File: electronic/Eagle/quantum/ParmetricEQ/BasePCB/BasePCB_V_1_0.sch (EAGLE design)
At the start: 62 parts, among them IC1 OP275_SOIC8, IC2 OP275_SOIC8, IC3 OP275_SOIC8, IC4 DAC084S085CIMM_NOPB, J1 90814-0204, J2 90814-0204, U1 THAT2181SO8-US, U2 THAT2181SO8-US, U3 THAT2181SO8-US

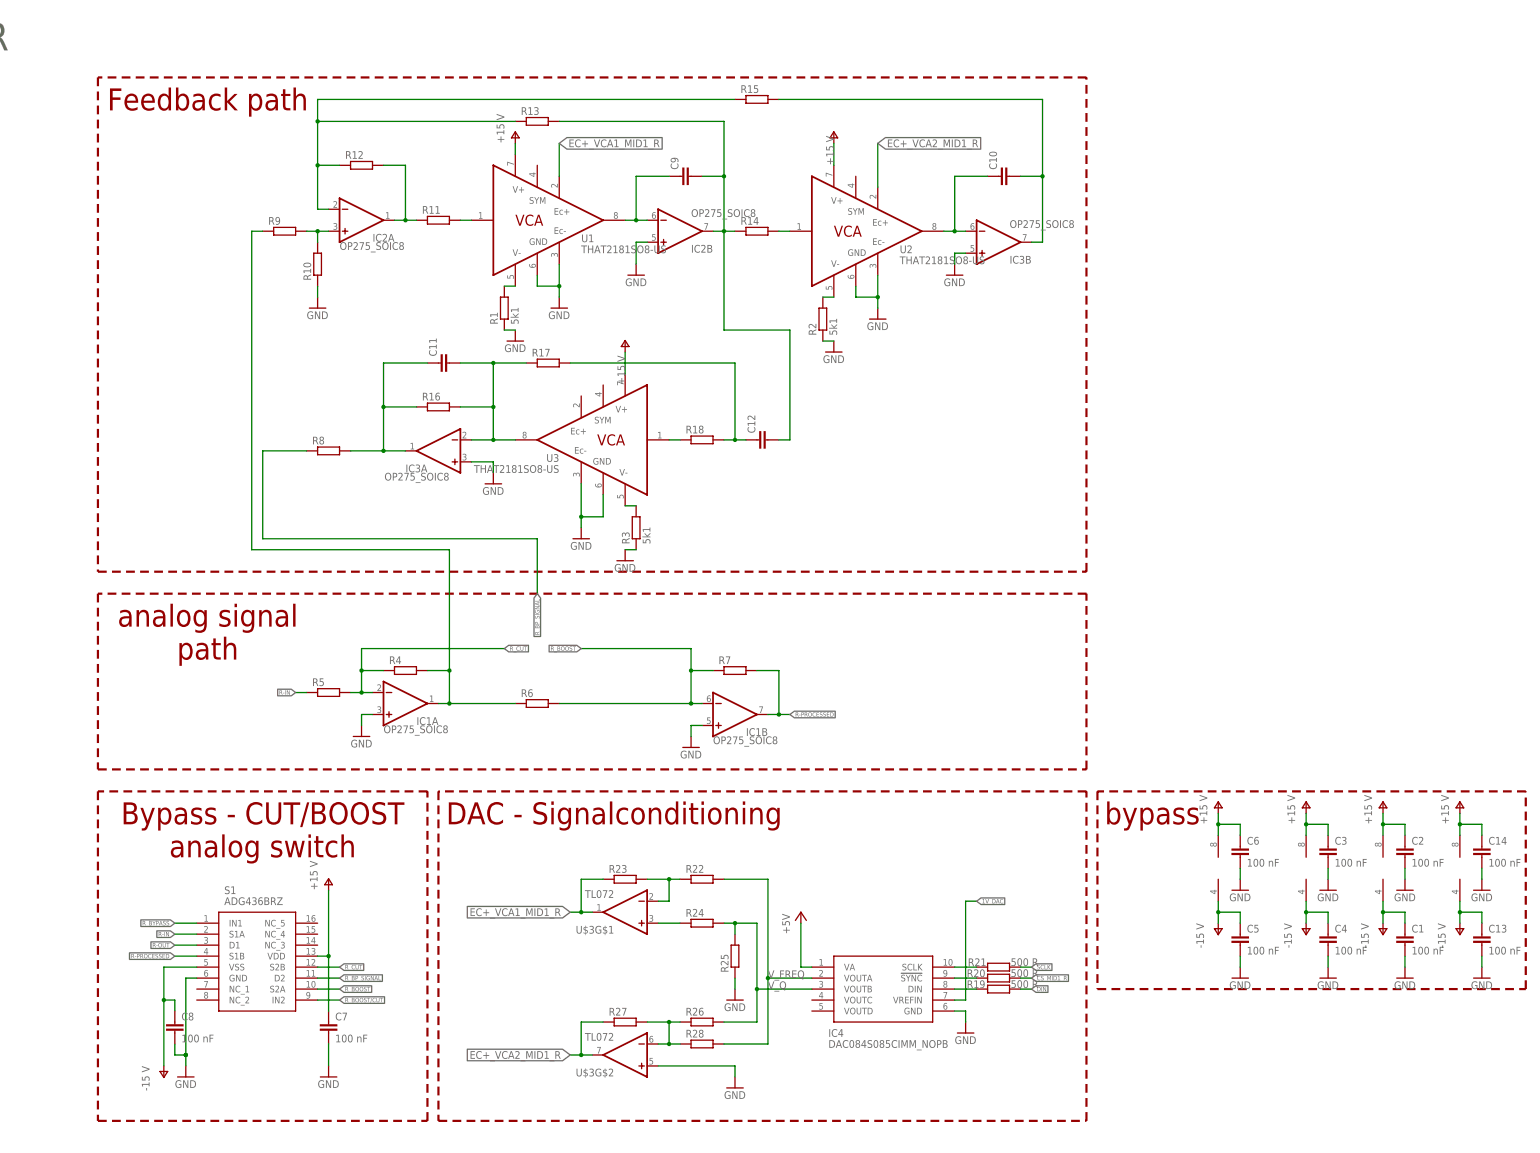
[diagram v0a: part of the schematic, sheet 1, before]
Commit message: updates ParametricEQ
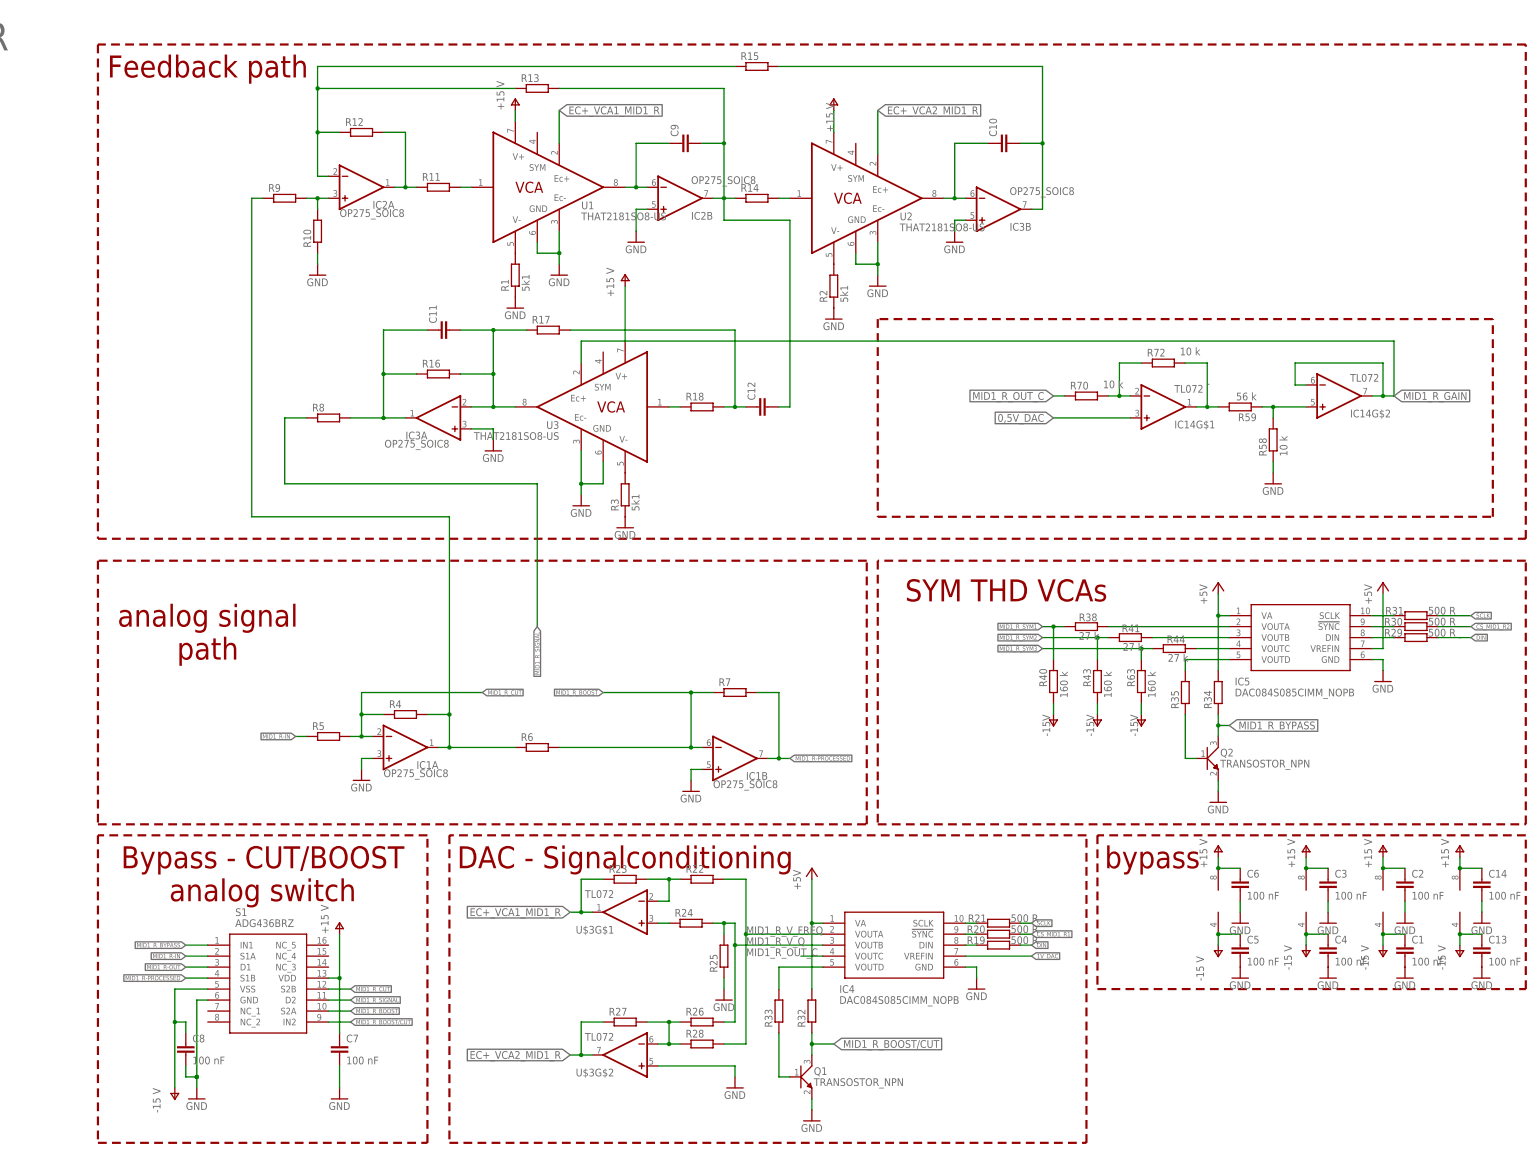
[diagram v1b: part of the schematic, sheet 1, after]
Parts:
- added C15, C16, C17: 100 nF, passive components:CAPACITOR_0603
- added C18: 10 uF, passive components:CAPACITOR_1206
- added I2C-CONN, PRG-CONN: 90814-0204, electro_mechanical:90814-0204
- added IC14: TL072, OP-AMPS:TL072
- added IC5: DAC084S085CIMM_NOPB, SPI:DAC084S085CIMM_NOPB
- added IC6: STM32F031K6T6, C_Sager_Bibliothek:STM32F031K6T6
- added J10, J3, J4, J5, J6, J7, J8, J9: 10018784-10210TLF, electro_mechanical:10018784-10210TLF
- added Q1, Q2: TRANSOSTOR_NPN, active components:TRANSOSTOR_NPN
- added R29, R30, R31: 500 R, passive components:RESISTOR_0603
- added R32, R33, R34, R35: (no value), passive components:RESISTOR_0603
- added R36, R37, R39: 10k, passive components:RESISTOR_0603
- added R38, R41, R44: 27 k, passive components:RESISTOR_0603
- added R40, R43, R63: 160 k, passive components:RESISTOR_0603
- added R58, R70, R72: 10 k, passive components:RESISTOR_0603
- added R59: 56 k, passive components:RESISTOR_0603
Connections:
- net R-IN renamed MID1_R-IN
- net R-OUT renamed MID1_R-OUT
- net R-PROCESSED renamed MID1_R-PROCESSED
- net R_BOOST renamed MID1_R_BOOST
- net R_BP_SIGNAL renamed MID1_R_SIGNAL
- net R_CUT renamed MID1_R_CUT
- net V_FREQ renamed MID1_R_V_FREQ
- net V_Q renamed MID1_R_V_Q
- removed net CS_MID1_R: R20.2
- removed net R_BOOST/CUT: S1.IN2
- removed net R_BYPASS: S1.IN1
- new net +3V3: C15.1, C16.1, C17.1, C18.1, I2C-CONN.3, IC6.VDDA, IC6.VDD_1, IC6.VDD_2
- new net .: IC14G$1.OUT, R59.2, R72.2
- new net ADRR.1: IC6.PF0-OSC_IN, R39.2
- new net ADRR.2: IC6.PF1-OSC_OUT, R36.2
- new net BOOT_0: IC6.BOOT0, R37.2
- new net CS_MID1_R1: R20.2, R30.2
- new net DIN1: R29.2
- new net I2C1_SCL: I2C-CONN.2, IC6.PB6
- new net I2C1_SDA: I2C-CONN.1, IC6.PA10
- new net MID1_R_BOOST/CUT: Q1.C, R32.1, S1.IN2
- new net MID1_R_BYPASS: Q2.C, R34.1, S1.IN1
- new net MID1_R_GAIN: IC14G$2.-IN, IC14G$2.OUT, U3.EC+
- new net MID1_R_OUT_C: IC4.VOUTC, R70.1
- new net MID1_R_SYM1: R38.1, R40.2
- new net MID1_R_SYM2: R41.1, R43.2
- new net MID1_R_SYM3: R44.1, R63.2
- new net N$24: IC5.DIN, R29.1
- new net N$25: IC5.!SYNC, R30.1
- new net N$26: IC4.VOUTD, R33.2
- new net N$27: IC5.SCLK, R31.1
- new net N$28: Q2.B, R35.1
- new net N$29: Q1.B, R33.1
- new net N$30: IC5.VOUTD, R35.2
- new net N$56: IC5.VOUTA, R38.2
- new net N$57: IC5.VOUTB, R41.2
- new net N$58: IC5.VOUTC, R44.2
- new net N$66: IC14G$2.+IN, R58.2, R59.1
- new net N$74: IC14G$1.-IN, R70.2, R72.1
- new net NRST: IC6.NRST, PRG-CONN.2
- new net SCLK1: R31.2
- new net SWCLK: IC6.PA14, PRG-CONN.1
- new net SWDIO: IC6.PA13, PRG-CONN.3
- net +5V: now also IC5.VA, IC5.VREFIN, R32.2, R34.2
- net 0,5V_DAC: now also IC14G$1.+IN
- net GND: now also C15.2, C16.2, C17.2, C18.2, I2C-CONN.4, IC5.GND, IC6.VSS_1, IC6.VSS_2, PRG-CONN.4, Q1.E, Q2.E, R36.1, R37.1, R39.1, R58.1
- net V-: now also R40.1, R43.1, R63.1
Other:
- note added: "SYM THD VCAs"
- moved on the sheet: C1, C10, C11, C12, C13, C14, C2, C3, C4, C5, C6, C7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

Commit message: split PCB in ParametricEQ
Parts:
- removed C1, C13, C14, C19, C2, C3, C4, C5, C6, C7, C8: 100 nF, passive components:CAPACITOR_0603
- removed C10, C11, C12, C9: (no value), passive components:CAPACITOR_0603
- removed C64: 10 uF, passive components:CAPACITOR_1206
- removed IC1, IC2, IC3: OP275_SOIC8, OP-AMPS:OP275_SOIC8
- removed IC14, U$1, U$2, U$3: TL072, OP-AMPS:TL072
- removed IC4, IC5: DAC084S085CIMM_NOPB, SPI:DAC084S085CIMM_NOPB
- removed Q1, Q2: TRANSOSTOR_NPN, active components:TRANSOSTOR_NPN
- removed R1, R2, R3: 5k1, passive components:RESISTOR_0603
- removed R10, R11, R12, R13, R14, R15, R16, R17, R18, R22, R23, R24, R25, R26, R27, R28, R32, R33, R34, R35, R4, R5, R6, R7, R8, R9: (no value), passive components:RESISTOR_0603
- removed R19, R20, R21, R29, R30, R31: 500 R, passive components:RESISTOR_0603
- removed R38, R41, R44: 27 k, passive components:RESISTOR_0603
- removed R40, R43, R63: 160 k, passive components:RESISTOR_0603
- removed R58, R60, R61, R67, R70, R72: 10 k, passive components:RESISTOR_0603
- removed R59: 56 k, passive components:RESISTOR_0603
- removed R68: 20 k, passive components:RESISTOR_0603
- removed S1: ADG436BRZ, analog switches:ADG436BRZ
- removed U1, U2, U3: THAT2181SO8-US, THAT_Library:THAT2181SO8-US
- removed Z1: ZENER_DIODE_BZT, passive components:ZENER_DIODE_BZT
- added C20, C22, C24, C26, C28, C30, C32, C34, C37, C39, C41, C43, C45, C47, C49: 10 uF, passive components:CAPACITOR_1206
- added C21, C23, C25, C27, C29, C31, C33, C35, C36, C38, C40, C42, C44, C46, C48, C50: 100 nF, passive components:CAPACITOR_0603
- added IC10, IC11, IC12, IC13, IC15, IC7, IC8, IC9: DAC084S085CIMM_NOPB, SPI:DAC084S085CIMM_NOPB
- added R42, R45, R46, R47, R48, R49, R50, R51, R52, R53, R54, R55, R56, R57, R62, R64, R65, R66, R69, R71, R73, R74, R75, R76: 500 R, passive components:RESISTOR_0603
- C15: value 100 nF -> 10 uF; device passive components:CAPACITOR_0603 -> passive components:CAPACITOR_1206
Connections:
- removed net .: IC14G$1.OUT, R59.2, R72.2
- removed net 0,5V_DAC: IC14G$1.+IN, U$2G$2.-IN, U$2G$2.OUT
- removed net 1V_DAC: IC4.VREFIN, U$2G$1.-IN, U$2G$1.OUT
- removed net 1V_DAC_UNBUFFERD: C19.1, C64.1, R61.2, R68.1, U$2G$1.+IN
- removed net 2V_DAC_REF: R67.1, R68.2, Z1.K
- removed net AGND: C19.2, C64.2, R60.1, Z1.A
- removed net CS_MID1_R1: R20.2, R30.2
- removed net DIN: R19.2
- removed net DIN1: R29.2
- removed net EC+_VCA1_MID1_R: R23.1, U$3G$1.OUT, U1.EC+
- removed net EC+_VCA2_MID1_R: R27.1, U$3G$2.OUT, U2.EC+
- removed net MID1_R-IN: J2.1, R5.1, S1.S1A
- removed net MID1_R-OUT: J2.2, S1.D1
- removed net MID1_R-PROCESSED: IC1B.OUT, R7.2, S1.S1B
- removed net MID1_R_BOOST: IC1B.-IN, R6.2, R7.1, S1.S2A
- removed net MID1_R_BOOST/CUT: Q1.C, R32.1, S1.IN2
- removed net MID1_R_BYPASS: Q2.C, R34.1, S1.IN1
- removed net MID1_R_CUT: IC1A.-IN, R4.1, R5.2, S1.S2B
- removed net MID1_R_GAIN: IC14G$2.-IN, IC14G$2.OUT, U3.EC+
- removed net MID1_R_OUT_C: IC4.VOUTC, R70.1
- removed net MID1_R_SIGNAL: R8.1, S1.D2
- removed net MID1_R_SYM1: R38.1, R40.2
- removed net MID1_R_SYM2: R41.1, R43.2
- removed net MID1_R_SYM3: R44.1, R63.2
- removed net MID1_R_V_FREQ: IC4.VOUTA, R22.2, R28.2
- removed net MID1_R_V_Q: IC4.VOUTB, R24.2, R25.2, R26.2
- removed net N$10: C12.2, C9.2, IC2B.OUT, R13.2, R14.1
- removed net N$11: R14.2, U2.IN
- removed net N$12: C10.1, IC3B.-IN, U2.OUT
- removed net N$13: C11.1, IC3A.OUT, R16.1, R8.2
- removed net N$14: C10.2, IC3B.OUT, R15.2
- removed net N$15: C11.2, IC3A.-IN, R16.2, R17.1, U3.OUT
- removed net N$16: R18.1, U3.IN
- removed net N$17: C12.1, R17.2, R18.2
- removed net N$18: IC4.DIN, R19.1
- removed net N$19: IC4.!SYNC, R20.1
- removed net N$20: IC4.SCLK, R21.1
- removed net N$21: R22.1, R23.2, U$3G$1.-IN
- removed net N$22: R24.1, U$3G$1.+IN
- removed net N$23: R26.1, R27.2, R28.1, U$3G$2.-IN
- removed net N$24: IC5.DIN, R29.1
- removed net N$25: IC5.!SYNC, R30.1
- removed net N$26: IC4.VOUTD, R33.2
- removed net N$27: IC5.SCLK, R31.1
- removed net N$28: Q2.B, R35.1
- removed net N$29: Q1.B, R33.1
- removed net N$30: IC5.VOUTD, R35.2
- removed net N$56: IC5.VOUTA, R38.2
- removed net N$57: IC5.VOUTB, R41.2
- removed net N$58: IC5.VOUTC, R44.2
- removed net N$66: IC14G$2.+IN, R58.2, R59.1
- removed net N$67: R60.2, R61.1, U$2G$2.+IN
- removed net N$74: IC14G$1.-IN, R70.2, R72.1
- removed net N$8: R11.2, U1.IN
- removed net N$9: C9.1, IC2B.-IN, U1.OUT
- removed net SCLK: R21.2
- removed net SCLK1: R31.2
- new net N$31: IC7.DIN, R42.1
- new net N$32: IC7.!SYNC, R45.1
- new net N$33: IC7.SCLK, R46.1
- new net N$34: IC7.VOUTA
- new net N$35: IC7.VOUTB
- new net N$36: IC7.VOUTC
- new net N$37: IC7.VOUTD
- new net N$38: IC8.DIN, R47.1
- new net N$39: IC8.!SYNC, R48.1
- new net N$40: IC8.SCLK, R49.1
- new net N$41: IC8.VOUTA
- new net N$42: IC8.VOUTB
- new net N$43: IC8.VOUTC
- new net N$44: IC8.VOUTD
- new net N$45: IC9.DIN, R50.1
- new net N$46: IC9.!SYNC, R51.1
- new net N$47: IC9.SCLK, R52.1
- new net N$48: IC9.VOUTA
- new net N$49: IC9.VOUTB
- new net N$50: IC9.VOUTC
- new net N$51: IC9.VOUTD
- new net N$52: IC10.DIN, R53.1
- new net N$53: IC10.!SYNC, R54.1
- new net N$54: IC10.SCLK, R55.1
- new net N$55: IC10.VOUTA
- new net N$59: IC10.VOUTB
- new net N$60: IC10.VOUTC
- new net N$61: IC10.VOUTD
- new net N$62: IC11.DIN, R56.1
- new net N$63: IC11.!SYNC, R57.1
- new net N$64: IC11.SCLK, R62.1
- new net N$65: IC11.VOUTA
- new net N$68: IC11.VOUTB
- new net N$69: IC11.VOUTC
- new net N$70: IC11.VOUTD
- new net N$71: IC12.DIN, R64.1
- new net N$72: IC12.!SYNC, R65.1
- new net N$73: IC12.SCLK, R66.1
- new net N$75: IC12.VOUTA
- new net N$76: IC12.VOUTB
- new net N$77: IC12.VOUTC
- new net N$78: IC12.VOUTD
- new net N$79: IC13.DIN, R69.1
- new net N$80: IC13.!SYNC, R71.1
- new net N$81: IC13.SCLK, R73.1
- new net N$82: IC13.VOUTA
- new net N$83: IC13.VOUTB
- new net N$84: IC13.VOUTC
- new net N$85: IC13.VOUTD
- new net N$86: IC15.DIN, R74.1
- new net N$87: IC15.!SYNC, R75.1
- new net N$88: IC15.SCLK, R76.1
- new net N$89: IC15.VOUTA
- new net N$90: IC15.VOUTB
- new net N$91: IC15.VOUTC
- new net N$92: IC15.VOUTD
- new net R-IN: J2.1
- new net R-OUT: J2.2
- net +3V3: no longer C15.1
- net +5V: now also C15.1, C20.1, C21.1, C22.1, C23.1, C24.1, C25.1, C26.1, C27.1, C28.1, C29.1, C30.1, C31.1, C32.1, C33.1, C34.1, C35.1, C36.1, C37.1, C38.1, C39.1, C40.1, C41.1, C42.1, C43.1, C44.1, C45.1, C46.1, C47.1, C48.1, C49.1, C50.1, IC10.VA, IC10.VREFIN, IC11.VA, IC11.VREFIN, IC12.VA, IC12.VREFIN, IC13.VA, IC13.VREFIN, IC15.VA, IC15.VREFIN, IC7.VA, IC7.VREFIN, IC8.VA, IC8.VREFIN, IC9.VA, IC9.VREFIN; no longer IC4.VA, IC5.VA, IC5.VREFIN, R32.2, R34.2
- net GND: now also C20.2, C21.2, C22.2, C23.2, C24.2, C25.2, C26.2, C27.2, C28.2, C29.2, C30.2, C31.2, C32.2, C33.2, C34.2, C35.2, C36.2, C37.2, C38.2, C39.2, C40.2, C41.2, C42.2, C43.2, C44.2, C45.2, C46.2, C47.2, C48.2, C49.2, C50.2, IC10.GND, IC11.GND, IC12.GND, IC13.GND, IC15.GND, IC7.GND, IC8.GND, IC9.GND; no longer C1.2, C13.2, C14.2, C2.2, C3.2, C4.2, C5.2, C6.2, C7.2, C8.2, IC1A.+IN, IC1B.+IN, IC2B.+IN, IC3A.+IN, IC3B.+IN, IC4.GND, IC5.GND, Q1.E, Q2.E, R1.1, R10.1, R2.1, R25.1, R3.1, R58.1, S1.GND, U$3G$2.+IN, U1.EC-, U1.GND, U2.EC-, U2.GND, U3.EC-, U3.GND
- net N$1: now also J9.B18; no longer R1.2, U1.V-
- net N$2: now also J4.B18; no longer R2.2, U2.V-
- net N$3: now also J3.B18; no longer R3.2, U3.V-
- net N$4: now also J8.B18; no longer IC2A.+IN, R10.2, R9.2
- net N$5: now also J7.B18; no longer IC1A.OUT, R4.2, R6.1, R9.1
- net N$6: now also J5.B18; no longer IC2A.-IN, R12.1, R13.1, R15.1
- net N$7: now also J6.B18; no longer IC2A.OUT, R11.1, R12.2
- net V+: now also J10.A1, J10.B1, J3.A1, J3.B1, J4.A1, J4.B1, J5.A1, J5.B1, J6.A1, J6.B1, J7.A1, J7.B1, J8.A1, J8.B1, J9.A1, J9.B1; no longer C14.1, C2.1, C3.1, C6.1, C7.1, IC1P.V+, IC2P.V+, IC3P.V+, R67.2, S1.VDD, U$3G$3.V+, U1.V+, U2.V+, U3.V+
- net V-: now also J10.A18, J10.B18, J3.A18, J4.A18, J5.A18, J6.A18, J7.A18, J8.A18, J9.A18; no longer C1.1, C13.1, C4.1, C5.1, C8.1, IC1P.V-, IC2P.V-, IC3P.V-, R40.1, R43.1, R63.1, S1.VSS, U$3G$3.V-
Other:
- note removed: "Bypass - CUT/BOOST analog switch"
- note removed: "DAC - Signalconditioning"
- note removed: "DAC Ref Voltages"
- note removed: "Feedback path"
- note removed: "MID1_R"
- note removed: "SYM THD VCAs"
- note removed: "analog signal path"
- note removed: "bypass"
